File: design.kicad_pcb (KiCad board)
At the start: 2 copper layers, 79 x 55 mm, 4 parts, among them J1 2601-3108, J2 2601-3108, J3 2601-3108, U1 ATtiny1616-S

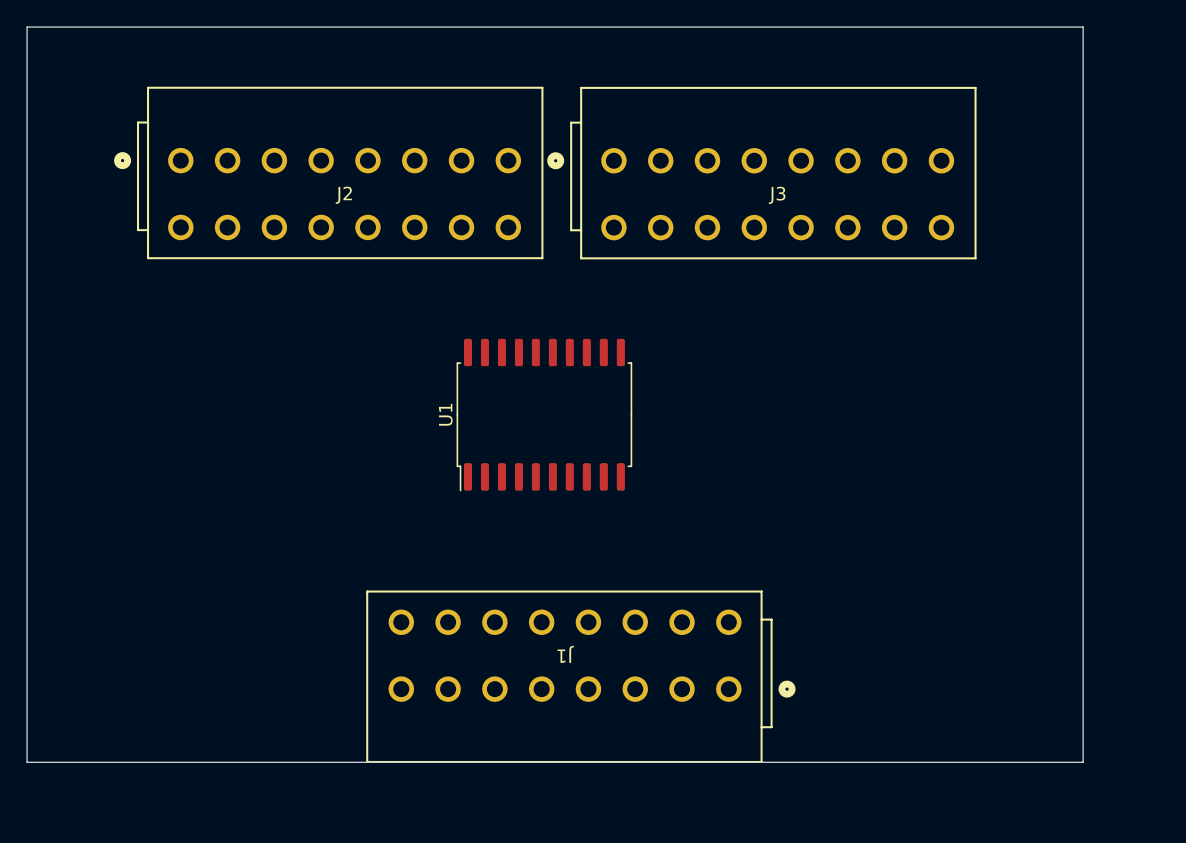
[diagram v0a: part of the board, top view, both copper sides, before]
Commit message: update
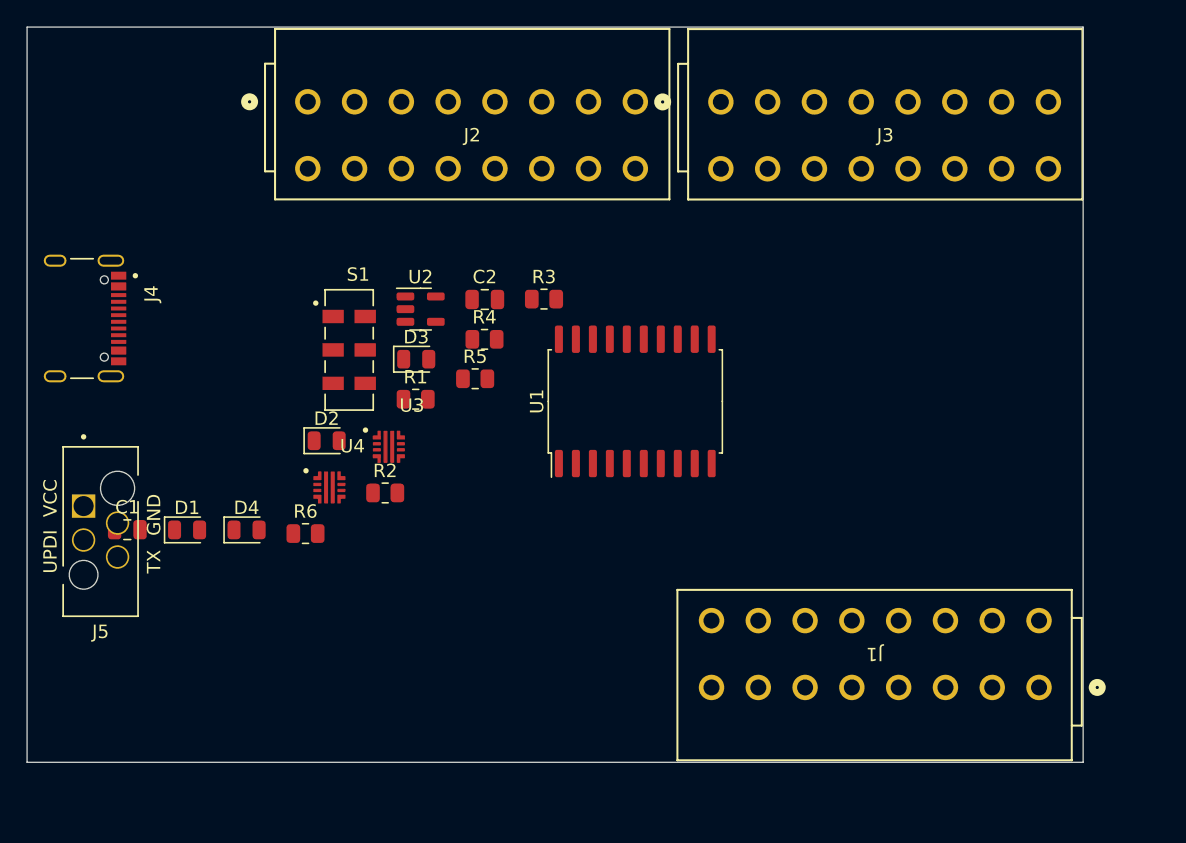
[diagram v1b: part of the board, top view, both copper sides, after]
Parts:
- added C1: 1uF, Capacitor_SMD:C_0805_2012Metric, F.Cu at (95.0, 103.2)
- added C2: 1uF, Capacitor_SMD:C_0805_2012Metric, F.Cu at (121.7, 86.0)
- added D1: 5V, LED_SMD:LED_0805_2012Metric, F.Cu at (99.5, 103.2)
- added D2: 3.3V, LED_SMD:LED_0805_2012Metric, F.Cu at (109.9, 96.5)
- added D3: 5V, LED_SMD:LED_0805_2012Metric, F.Cu at (116.6, 90.4)
- added D4: 3.3V, LED_SMD:LED_0805_2012Metric, F.Cu at (103.9, 103.2)
- added J4: TYPE-C-31-M-12, Snapeda:TYPE-C-31-M-12_HRO_TYPE-C-31-M-12, F.Cu at (89.6, 87.4)
- added J5: SKEDD-UPDI-4, Connector_custom:SKEDD-UPDI-4, F.Cu at (93.0, 103.3)
- added R1: 5.1k, Resistor_SMD:R_0805_2012Metric, F.Cu at (116.6, 93.4)
- added R2: 5.1k, Resistor_SMD:R_0805_2012Metric, F.Cu at (114.3, 100.5)
- added R3: 330, Resistor_SMD:R_0805_2012Metric, F.Cu at (126.2, 86.0)
- added R4: 330, Resistor_SMD:R_0805_2012Metric, F.Cu at (121.7, 89.0)
- added R5: 330, Resistor_SMD:R_0805_2012Metric, F.Cu at (121.0, 91.9)
- added R6: 330, Resistor_SMD:R_0805_2012Metric, F.Cu at (108.3, 103.5)
- added S1: JS202011JCQN, Snapeda:SW_JS202011JCQN, F.Cu at (111.6, 89.8)
- added U2: AP2112K-3.3, Package_TO_SOT_SMD:SOT-23-5, F.Cu at (116.9, 86.7)
- added U3: LM73100RPWR, Snapeda:LM73100RPWR_IC_LM73100RPWR, F.Cu at (114.6, 97.0)
- added U4: LM73100RPWR, Snapeda:LM73100RPWR_IC_LM73100RPWR, F.Cu at (110.1, 100.0)
- moved J1 23.2 mm to (163.2, 115.0)
- moved J2 10.5 mm to (108.5, 71.2)
- moved J3 9.13 mm to (139.4, 71.2)
- moved U1 6.87 mm to (133.0, 93.6)
